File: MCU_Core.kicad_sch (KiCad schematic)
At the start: 16 parts, among them U1 STM32F405RGTx

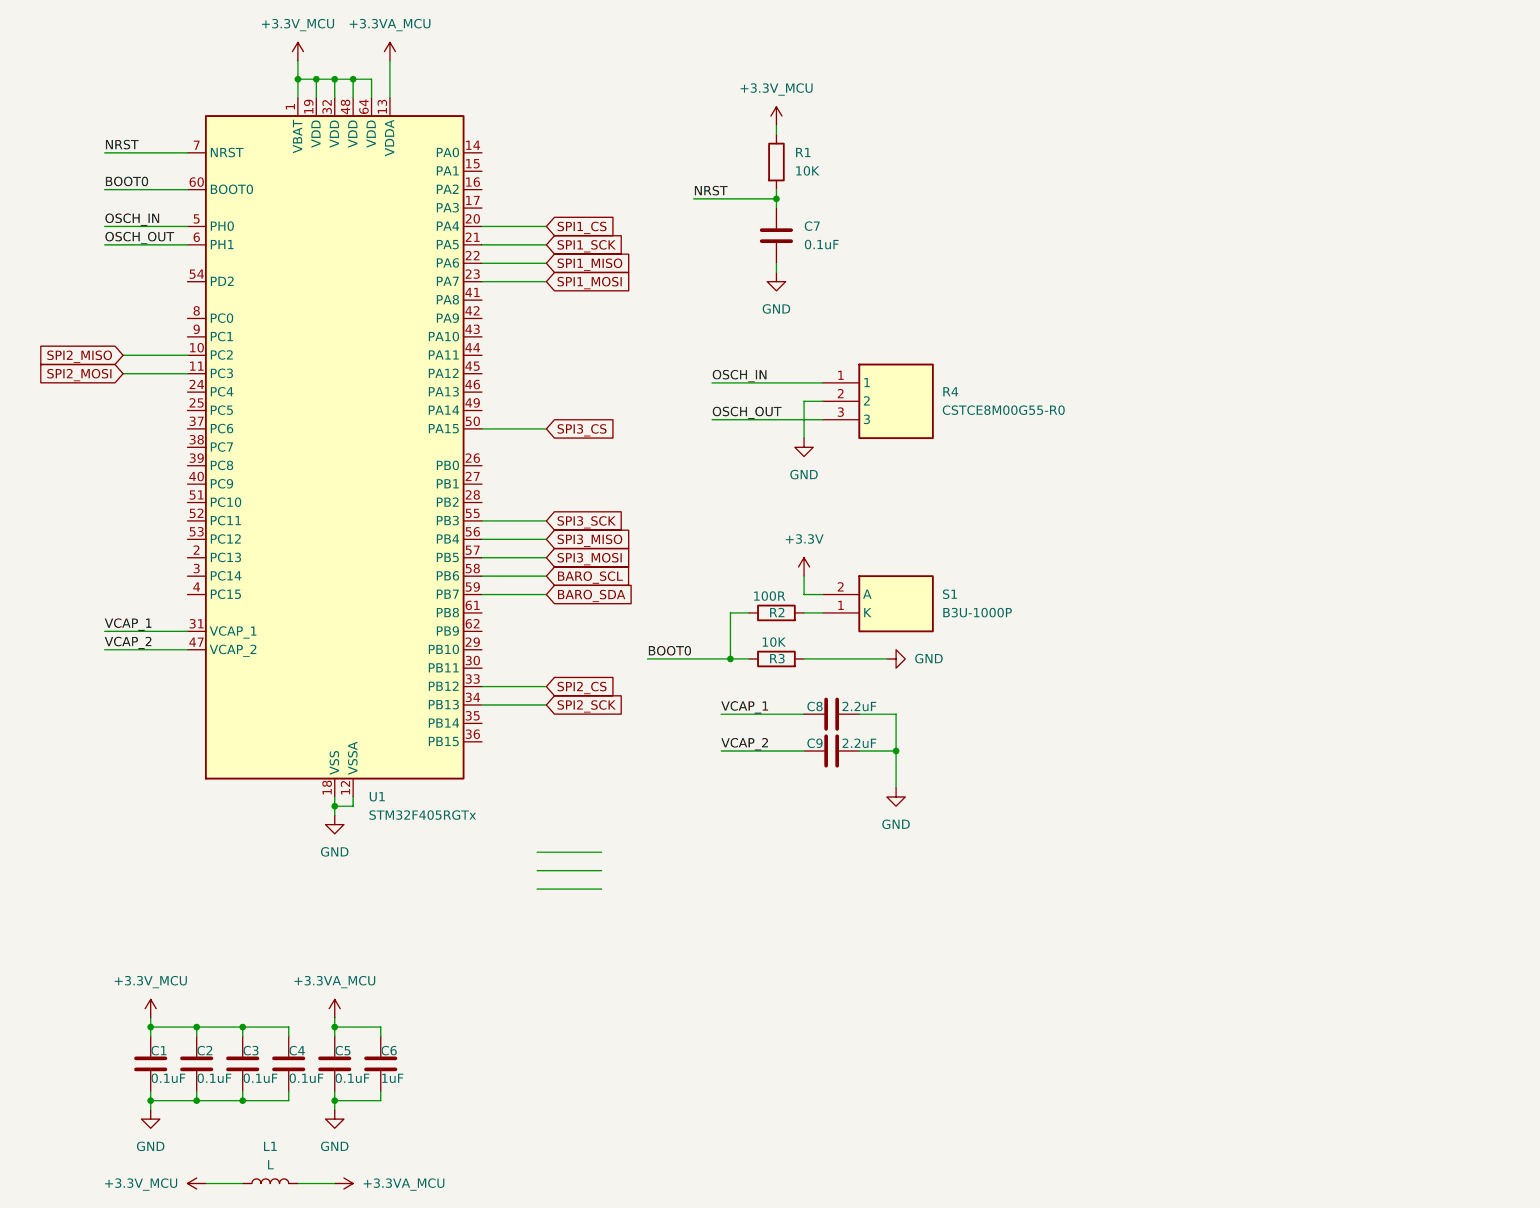
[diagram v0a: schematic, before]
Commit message: Finished SCH
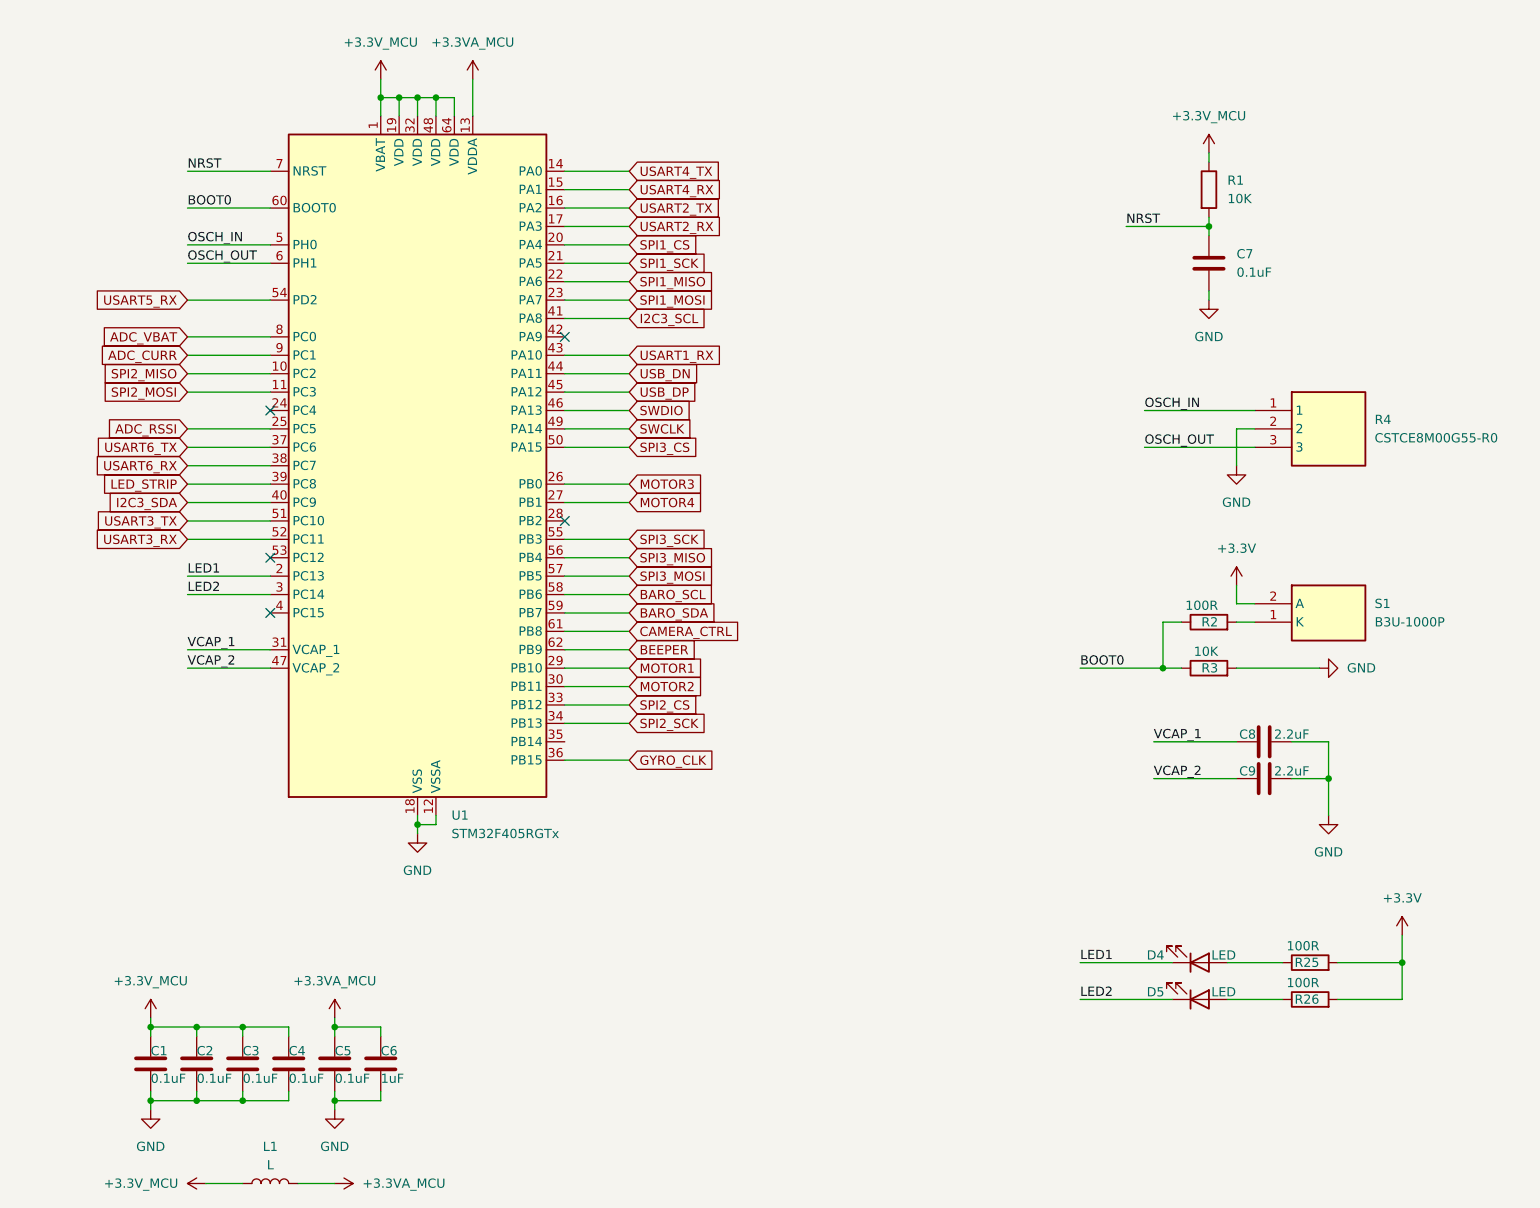
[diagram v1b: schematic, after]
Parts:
- added D4, D5: LED, LED_SMD:LED_0603_1608Metric, symbol Device:LED
- added R25, R26: 100R, Resistor_SMD:R_0402_1005Metric, symbol Library:R
- C1, C2, C3, C4, C5, C6, C7, C8, C9: footprint (none) -> Capacitor_SMD:C_0402_1005Metric
- L1: footprint (none) -> Inductor_SMD:L_0603_1608Metric
- R1: footprint (none) -> Resistor_SMD:R_0402_1005Metric
- R2, R3: footprint Resistor_SMD:R_0603_1608Metric -> Resistor_SMD:R_0402_1005Metric
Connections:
- net +3.3V: now also R25.2, R26.2
- net USART4_TX: now reaches U1.14 (PA0)
- net USART4_RX: now reaches U1.15 (PA1)
- net USART2_TX: now reaches U1.16 (PA2)
- net USART2_RX: now reaches U1.17 (PA3)
- net LED1: now reaches U1.2 (PC13)
- net LED1: now also D4.1 (K)
- net ADC_RSSI: now reaches U1.25 (PC5)
- net MOTOR3: now reaches U1.26 (PB0)
- net MOTOR4: now reaches U1.27 (PB1)
- net MOTOR1: now reaches U1.29 (PB10)
- net LED2: now reaches U1.3 (PC14)
- net LED2: now also D5.1 (K)
- net MOTOR2: now reaches U1.30 (PB11)
- net GYRO_CLK: now reaches U1.36 (PB15)
- net USART6_TX: now reaches U1.37 (PC6)
- net USART6_RX: now reaches U1.38 (PC7)
- net LED_STRIP: now reaches U1.39 (PC8)
- net I2C3_SDA: now reaches U1.40 (PC9)
- net I2C3_SCL: now reaches U1.41 (PA8)
- net USART1_RX: now reaches U1.43 (PA10)
- net USB_DN: now reaches U1.44 (PA11)
- net USB_DP: now reaches U1.45 (PA12)
- net SWDIO: now reaches U1.46 (PA13)
- net SWCLK: now reaches U1.49 (PA14)
- net USART3_TX: now reaches U1.51 (PC10)
- net USART3_RX: now reaches U1.52 (PC11)
- net USART5_RX: now reaches U1.54 (PD2)
- net CAMERA_CTRL: now reaches U1.61 (PB8)
- net BEEPER: now reaches U1.62 (PB9)
- net ADC_VBAT: now reaches U1.8 (PC0)
- net ADC_CURR: now reaches U1.9 (PC1)
- new net: D5.2 (A), R26.1
- new net: D4.2 (A), R25.1
- no-connect marks 0 -> 5
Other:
- moved on the sheet: C7, C8, C9, R1, R2, R3, R4, S1, U1
